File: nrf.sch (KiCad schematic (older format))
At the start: 9 parts, among them J2 Conn_01x05, SW1 UP, SW2 MID, SW3 DWN, U1 BLYST-NRF52832-NANO, U2 Oled_128x64_SSD1306

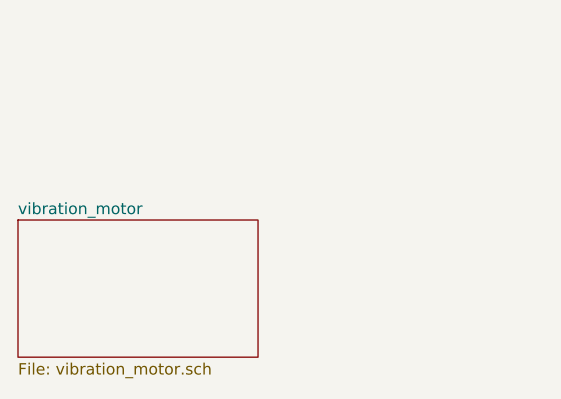
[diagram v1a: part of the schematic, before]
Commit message: New PCB's
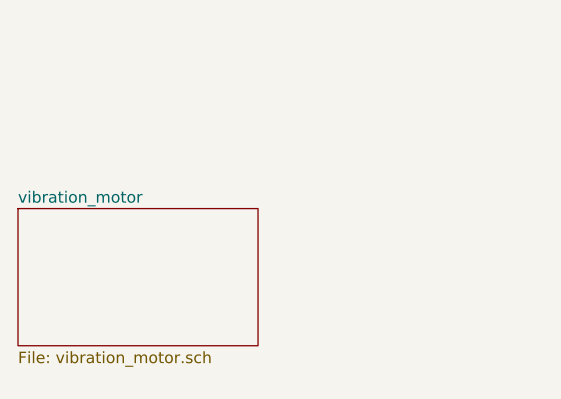
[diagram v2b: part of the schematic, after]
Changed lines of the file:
@@
 	8100 2850 7200 2850
 $Sheet
-S 650  7000 1050 600
+S 650  6950 1050 600
 U 5D059B17
 F0 "vibration_motor" 50
